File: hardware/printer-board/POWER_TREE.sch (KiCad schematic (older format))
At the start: 0 parts

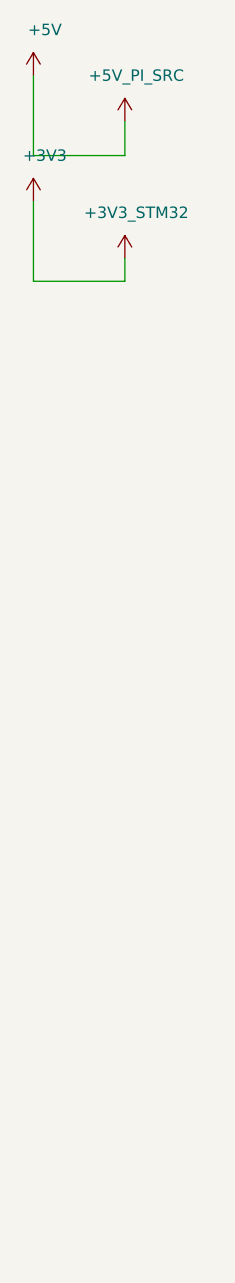
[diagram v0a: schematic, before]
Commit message: update,
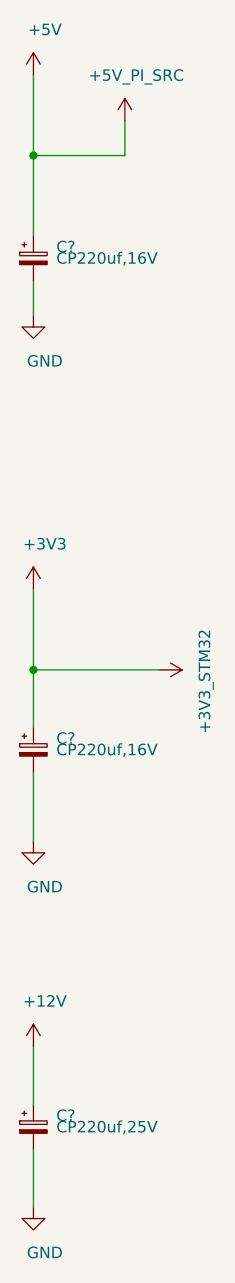
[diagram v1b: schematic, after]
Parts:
- added C?: CP220uf,25V, Capacitor_SMD:CP_Elec_8x10.5, symbol taobao-cp:CP220uf,25V
- added C? (x2): CP220uf,16V, Capacitor_SMD:CP_Elec_6.3x7.7, symbol taobao-cp:CP220uf,16V
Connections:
- net +3V3: now also C?.1
- net +5V: now also C?.1
- new net +12V: C?.1
- new net GND: C?.2, C?.2, C?.2
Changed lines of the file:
@@
 $Descr A4 11693 8268
 encoding utf-8
-Sheet 21 35
+Sheet 19 34
 Title ""
 Date ""
@@
 L power:+3V3 #PWR088
 U 1 1 5CC75BDD
-P 1550 1750
-F 0 "#PWR088" H 1550 1600 50  0001 C CNN
-F 1 "+3V3" H 1600 1950 50  0000 C CNN
-F 2 "" H 1550 1750 50  0001 C CNN
-F 3 "" H 1550 1750 50  0001 C CNN
-	1    1550 1750
+P 1550 3450
+F 0 "#PWR088" H 1550 3300 50  0001 C CNN
+F 1 "+3V3" H 1600 3650 50  0000 C CNN
+F 2 "" H 1550 3450 50  0001 C CNN
+F 3 "" H 1550 3450 50  0001 C CNN
+	1    1550 3450
 	1    0    0    -1
 $EndComp
@@
 L taobao-components:+3V3_STM32 #PWR089
 U 1 1 5CC75CBC
-P 1950 2000
-F 0 "#PWR089" H 1950 1850 50  0001 C CNN
-F 1 "+3V3_STM32" H 2000 2200 50  0000 C CNN
-F 2 "" H 1950 2000 50  0001 C CNN
-F 3 "" H 1950 2000 50  0001 C CNN
-	1    1950 2000
-	1    0    0    -1
+P 2100 3800
+F 0 "#PWR089" H 2100 3650 50  0001 C CNN
+F 1 "+3V3_STM32" H 2150 4000 50  0000 C CNN
+F 2 "" H 2100 3800 50  0001 C CNN
+F 3 "" H 2100 3800 50  0001 C CNN
+	1    2100 3800
+	0    1    1    0
 $EndComp
 Wire Wire Line
-	1550 1750 1550 2100
-Wire Wire Line
-	1550 2100 1950 2100
-Wire Wire Line
-	1950 2100 1950 2000
+	1550 3450 1550 3800
 $Comp
 L taobao-components:+5V_PI_SRC #PWR087
@@
 Wire Wire Line
 	1950 1550 1950 1400
+$Comp
+L power:+12V #PWR?
+U 1 1 5CCA90B1
+P 1550 5450
+F 0 "#PWR?" H 1550 5300 50  0001 C CNN
+F 1 "+12V" H 1600 5650 50  0000 C CNN
+F 2 "" H 1550 5450 50  0001 C CNN
+F 3 "" H 1550 5450 50  0001 C CNN
+	1    1550 5450
+	1    0    0    -1
+$EndComp
+$Comp
+L taobao-cp:CP220uf,25V C?
+U 1 1 5CCA916D
+P 1550 5800
+F 0 "C?" H 1650 5850 50  0000 L CNN
+F 1 "CP220uf,25V" H 1650 5800 50  0000 L CNN
+F 2 "Capacitor_SMD:CP_Elec_8x10.5" H 1550 5800 50  0001 C CNN
+F 3 "~" H 1550 5800 50  0001 C CNN
+	1    1550 5800
+	1    0    0    -1
+$EndComp
+$Comp
+L power:GND #PWR?
+U 1 1 5CCA920F
+P 1550 6150
+F 0 "#PWR?" H 1550 5900 50  0001 C CNN
+F 1 "GND" H 1600 5950 50  0000 C CNN
+F 2 "" H 1550 6150 50  0001 C CNN
+F 3 "" H 1550 6150 50  0001 C CNN
+	1    1550 6150
+	1    0    0    -1
+$EndComp
+Wire Wire Line
+	1550 5450 1550 5700
+Wire Wire Line
+	1550 5900 1550 6150
+Wire Wire Line
+	1550 3800 2100 3800
+$Comp
+L taobao-cp:CP220uf,16V C?
+U 1 1 5CCA9514
+P 1550 4150
+F 0 "C?" H 1650 4200 50  0000 L CNN
+F 1 "CP220uf,16V" H 1650 4150 50  0000 L CNN
+F 2 "Capacitor_SMD:CP_Elec_6.3x7.7" H 1550 4150 50  0001 C CNN
+F 3 "~" H 1550 4150 50  0001 C CNN
+	1    1550 4150
+	1    0    0    -1
+$EndComp
+$Comp
+L power:GND #PWR?
+U 1 1 5CCA95A1
+P 1550 4550
+F 0 "#PWR?" H 1550 4300 50  0001 C CNN
+F 1 "GND" H 1600 4350 50  0000 C CNN
+F 2 "" H 1550 4550 50  0001 C CNN
+F 3 "" H 1550 4550 50  0001 C CNN
+	1    1550 4550
+	1    0    0    -1
+$EndComp
+Wire Wire Line
+	1550 4250 1550 4550
+Wire Wire Line
+	1550 4050 1550 3800
+Connection ~ 1550 3800
+$Comp
+L taobao-cp:CP220uf,16V C?
+U 1 1 5CCA97CF
+P 1550 2000
+F 0 "C?" H 1650 2050 50  0000 L CNN
+F 1 "CP220uf,16V" H 1650 2000 50  0000 L CNN
+F 2 "Capacitor_SMD:CP_Elec_6.3x7.7" H 1550 2000 50  0001 C CNN
+F 3 "~" H 1550 2000 50  0001 C CNN
+	1    1550 2000
+	1    0    0    -1
+$EndComp
+Wire Wire Line
+	1550 1550 1550 1900
+Connection ~ 1550 1550
+$Comp
+L power:GND #PWR?
+U 1 1 5CCA998F
+P 1550 2250
+F 0 "#PWR?" H 1550 2000 50  0001 C CNN
+F 1 "GND" H 1600 2050 50  0000 C CNN
+F 2 "" H 1550 2250 50  0001 C CNN
+F 3 "" H 1550 2250 50  0001 C CNN
+	1    1550 2250
+	1    0    0    -1
+$EndComp
+Wire Wire Line
+	1550 2250 1550 2100
 $EndSCHEMATC
